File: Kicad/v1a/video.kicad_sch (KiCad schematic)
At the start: 30 parts, among them U10 74HC590A, U11 74HC590A, U12 74HC574, U13 74HC165, U14 74HC157, U15 74HC574, U7 74HC138, U8 SST39SF, U9 74HC574

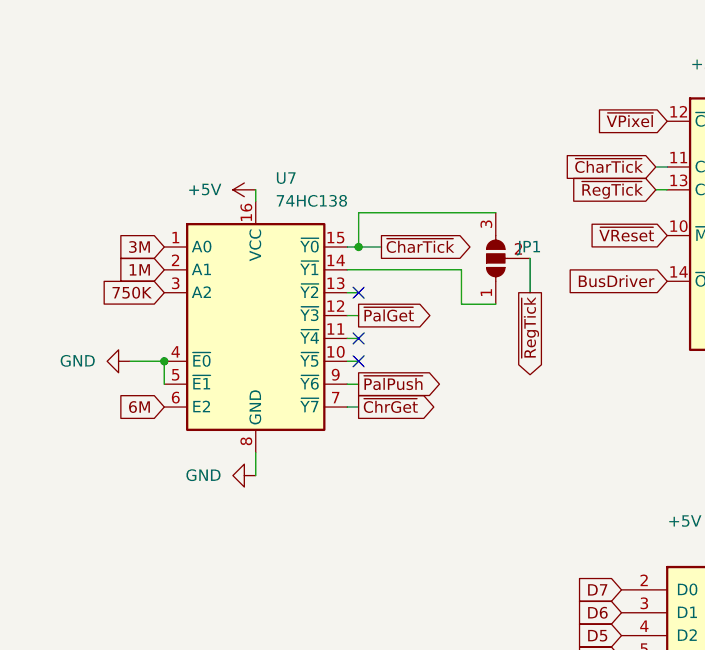
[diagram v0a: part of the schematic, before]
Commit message: v1a update
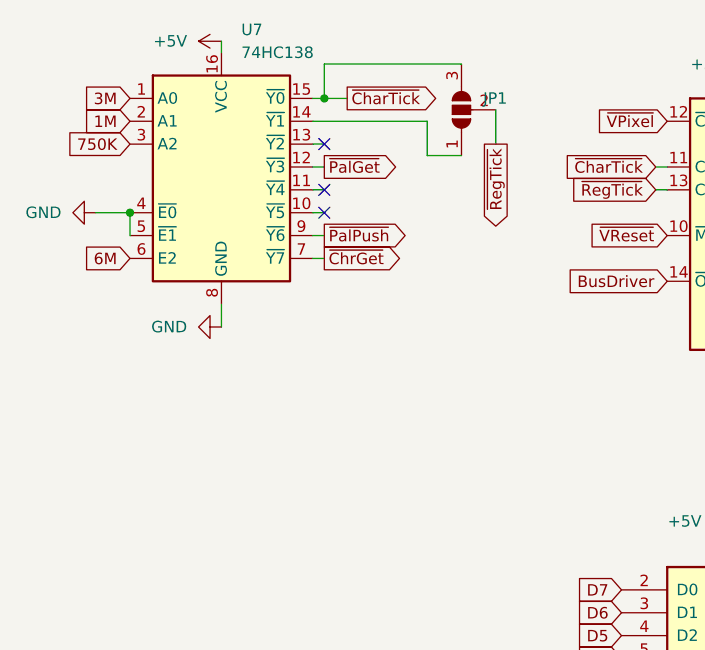
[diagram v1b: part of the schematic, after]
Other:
- moved on the sheet: JP1, U7
